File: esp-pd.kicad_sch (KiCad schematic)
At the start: 84 parts, among them J1 USB C Power, J2 USB C Data, J3 Power Out, J4 ESP PD Board pins, Q1 IRF7416, Q2 MMBT3904, SW1 Boot, SW2 Reset, SW3 Up, SW4 Down, SW5 VBUS Switch, U1 ESP32-C3, U2 FUSB302MPX, U3 TPD4E05U06DQA, U4 ME6217C33M5G, U5 MP9943GQ-Z, Y1 40 MHz

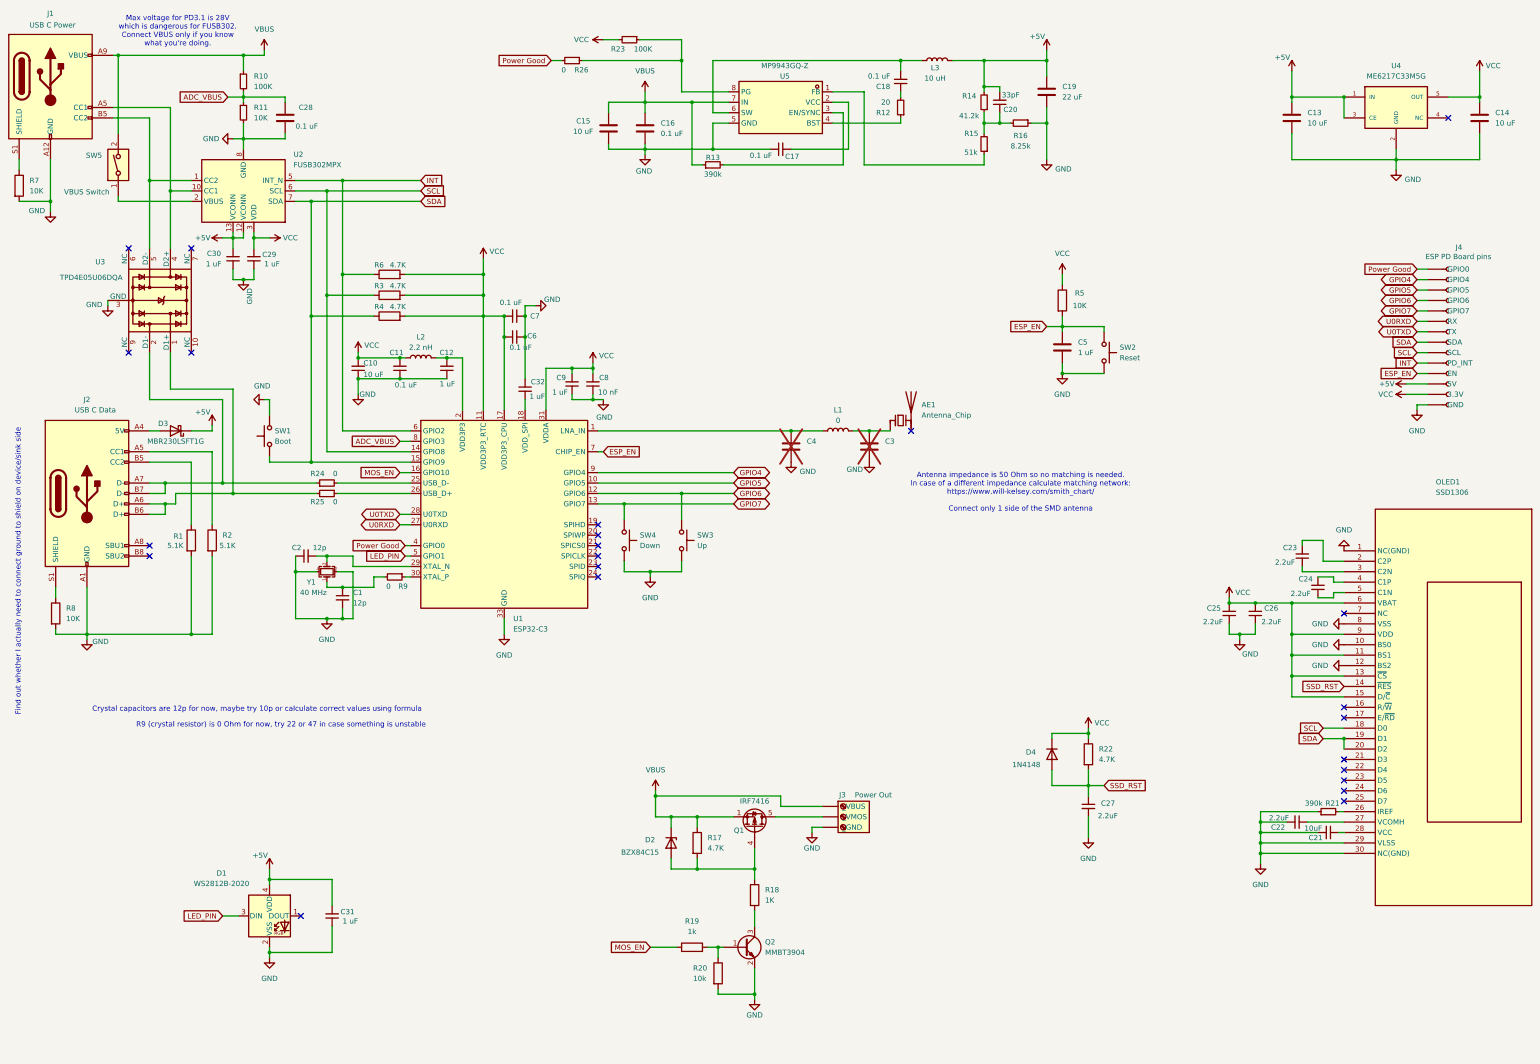
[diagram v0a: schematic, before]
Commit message: refactored
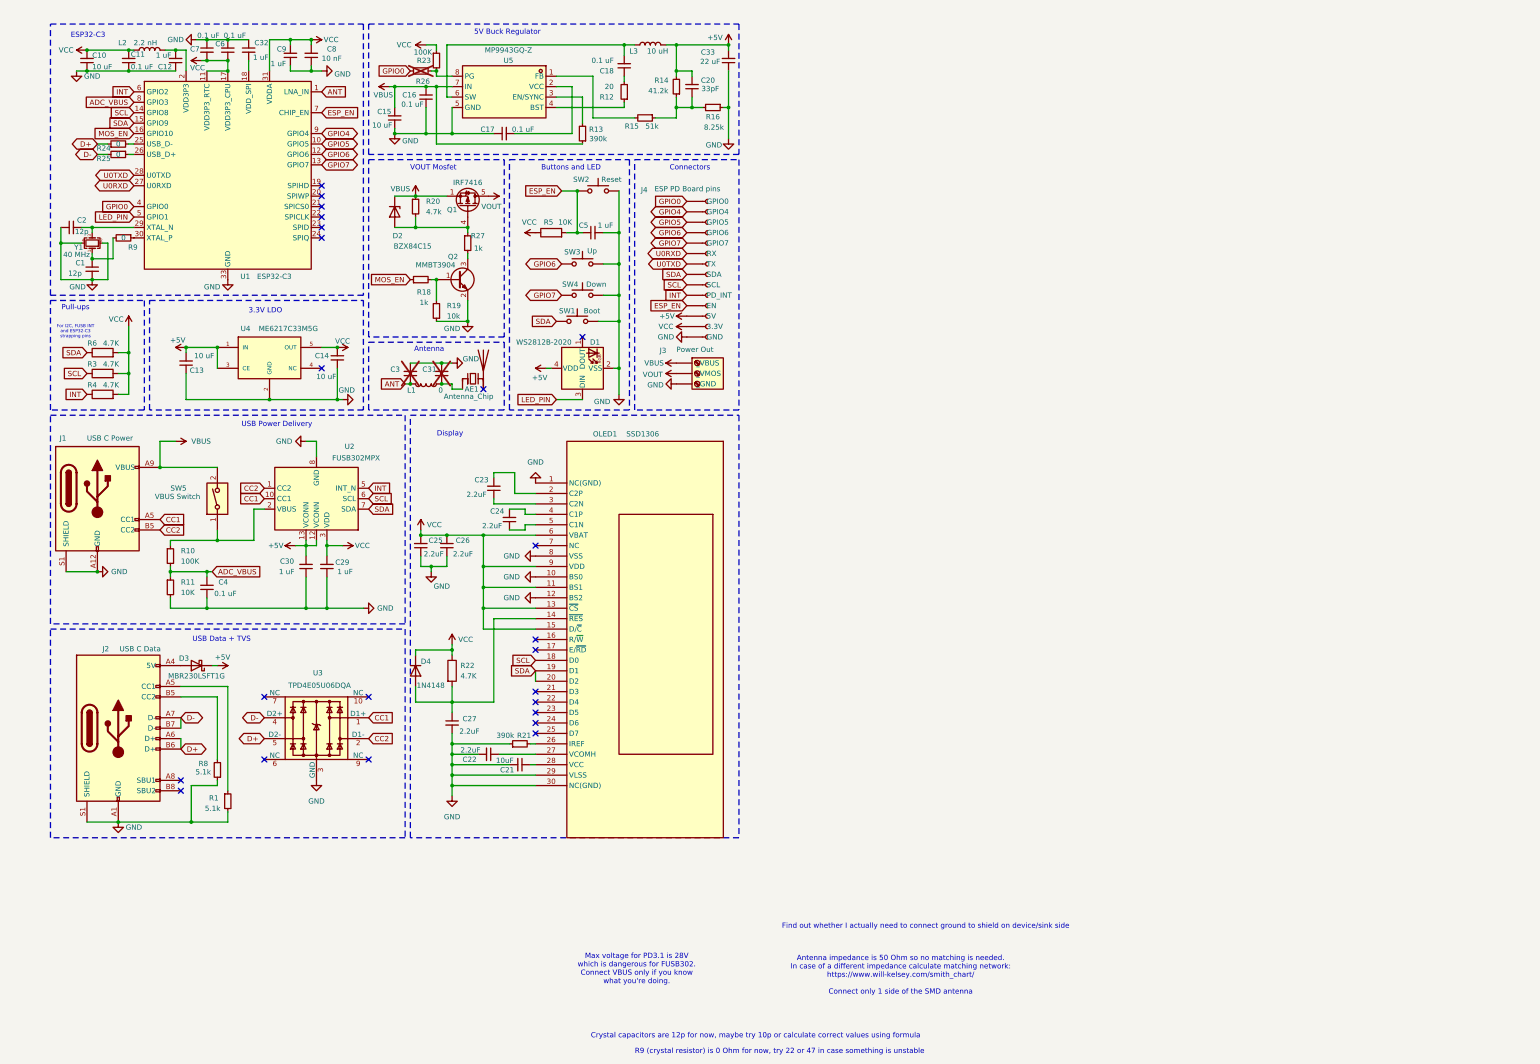
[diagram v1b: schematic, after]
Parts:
- removed C13, C14, C15: 10 uF, symbol Device:C
- removed C16, C28: 0.1 uF, symbol Device:C
- removed C19: 22 uF, symbol Device:C
- removed C3, C4: C, symbol Device:C
- removed C5: 1 uF, symbol Device:C
- removed R1, R2: 5.1K, symbol Device:R
- removed R17: 4.7K, symbol Device:R
- removed R18: 1K, symbol Device:R
- removed R19: 1k, symbol Device:R
- removed R20: 10k, symbol Device:R
- removed R7, R8: 10K, symbol Device:R
- added C13, C14, C15: 10 uF, symbol Device:C_Small
- added C16, C4: 0.1 uF, symbol Device:C_Small
- added C3: ~, symbol Device:C_Small
- added C33: 22 uF, symbol Device:C_Small
- added C5: 1 uF, symbol Device:C_Small
- added R1, R8: 5.1k, symbol Device:R_Small
- added R18, R27: 1k, symbol Device:R_Small
- added R19: 10k, symbol Device:R_Small
- added R20: 4.7k, symbol Device:R_Small
- C31: value 1 uF -> ~; now not fitted
- R26: now not fitted
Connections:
- net +5V: now also C13.2, C33.2; no longer C31.2
- net ADC_VBUS: now also C4.2
- net ESP_EN: now also C5.1
- net GND: now also C31.2, J1.S1 (SHIELD), J2.S1 (SHIELD), C13.1, C14.1, C15.1, C16.1, C3.2, C33.1, C4.1, C5.2, R1.2, R19.1, R8.1; no longer C31.1
- net INT: now also R4.1; no longer R6.1
- net MOS_EN: now also R18.1
- net SDA: now also R6.1; no longer R4.1
- net VBUS: now also C15.2, C16.2, R20.1; no longer R10.1
- net VCC: now also R23.1, C14.2; no longer R23.2
- net at L1.1: now also AE1.1 (FEED), C31.1; no longer U1.1 (LNA_IN)
- net at SW5.1, U2.2 (VBUS): now also R10.1
- net D-: now reaches J2.A7 (D-), J2.B7 (D-)
- net D-: now also R25.2, U3.4 (D2+); no longer R24.1, U3.2 (D1-)
- net at Q2.1 (B): now also R18.2, R19.2
- net D+: now reaches J2.A6 (D+), J2.B6 (D+)
- net D+: now also R24.1, U3.5 (D2-); no longer R25.2, U3.1 (D1+)
- net CC1: now reaches J1.A5 (CC1), U2.10 (CC1), U2.11 (CC1)
- net CC1: now also U3.1 (D1+); no longer U3.4 (D2+)
- net CC2: now reaches J1.B5 (CC2), U2.1 (CC2), U2.14 (CC2)
- net CC2: now also U3.2 (D1-); no longer U3.5 (D2-)
- net ANT: now reaches L1.2
- net ANT: now also U1.1 (LNA_IN), C3.1; no longer AE1.1 (FEED)
- net at D2.1 (A), Q1.4 (G): now also R20.2, R27.1
- net at U5.1 (FB): now also R15.2; no longer R15.1
- net at R26.1, U5.8 (PG): now also R23.2; no longer R23.1
- net at J2.B5 (CC2): now also R8.2
- net VOUT: now reaches J3.2 (_VMOS), Q1.5 (D), Q1.6 (D), Q1.7 (D), Q1.8 (D)
- net at J2.A5 (CC1): now also R1.1
- net at C20.1, R14.1, R16.2: now also R15.1; no longer R15.2
- net at Q2.3 (C): now also R27.2
- net Power Good renamed GPIO0
- net SSD_RST: no longer names the net of C27.1, D4.2 (A), OLED1.14 (~{RES}), R22.2
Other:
- note added: "3.3V LDO"
- note added: "5V Buck Regulator"
- note added: "Antenna"
- note added: "Buttons and LED"
- note added: "Connectors"
- note added: "Display"
- note added: "ESP32-C3"
- note added: "For I2C, FUSB INT and ESP32-C3 strapping pins"
- note added: "Pull-ups"
- note added: "USB Data + TVS"
- note added: "USB Power Delivery"
- note added: "VOUT Mosfet"
- moved on the sheet: AE1, C1, C10, C11, C12, C17, C18, C2, C20, C21, C22, C23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
